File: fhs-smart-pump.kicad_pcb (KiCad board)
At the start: 2 copper layers, 92 x 87 mm, 27 parts, among them J1 Barrel_Jack_Switch, J2 Conn_01x02, J3 Screw_Terminal_01x02, J5 Screw_Terminal_01x07, K1 G5NB, K2 G5NB, Q1 2SA1015, Q2 2SA1015, U1 LM2596T-5, U2 PC817, U3 ESP32-C3_SUPERMINI_TH, U4 PC817

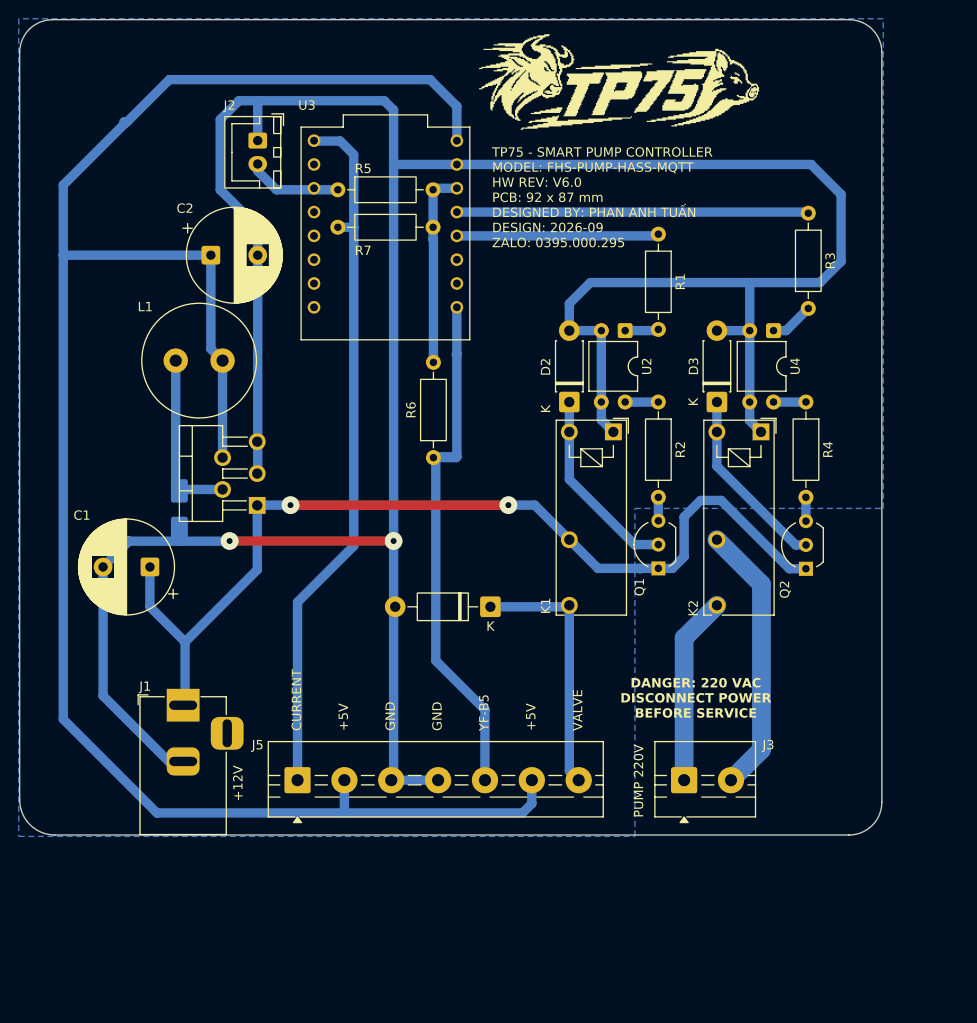
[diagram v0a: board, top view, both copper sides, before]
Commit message: cập nhật cơ khí pcb và báo cáo kiểm tra drc
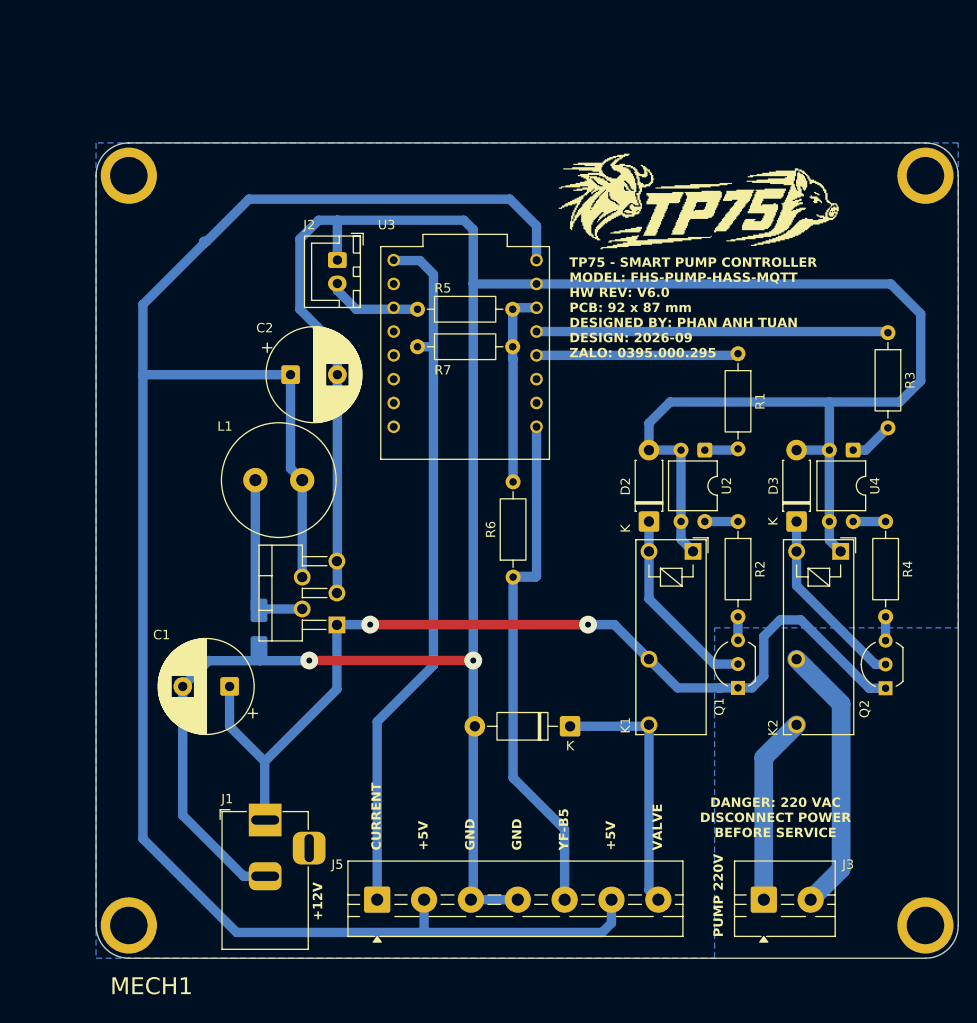
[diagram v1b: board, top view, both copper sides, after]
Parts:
- added MECH1: LK-PLC02_92x87, , F.Cu at (53.8, 150.0)
- moved ? 15.3 mm to (118.0, 69.2)
- moved C1 15.3 mm to (68.0, 121.0)
- moved C2 15.3 mm to (74.5, 87.7)
- moved D1 15.3 mm to (71.1, 114.9)
- moved D2 15.3 mm to (112.8, 103.4)
- moved D3 15.3 mm to (128.5, 103.4)
- moved D4 15.3 mm to (104.3, 125.2)
- moved J2 15.3 mm to (79.5, 75.5)
- moved J3 15.3 mm to (125.0, 143.8)
- moved J5 15.3 mm to (83.8, 143.8)
- moved K1 15.3 mm to (117.5, 106.6)
- moved L1 15.3 mm to (70.8, 99.0)
- moved Q1 15.3 mm to (122.2, 121.2)
- moved Q2 15.3 mm to (138.0, 121.2)
- moved R1 15.3 mm to (122.2, 85.5)
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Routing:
- net +12V: track 104.1 -> 103.5 mm
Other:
- outline, holes or cut-outs redrawn
- board text added: "TP75 - SMART PUMP CONTROLLER MODEL: FHS-PUMP-HASS-MQTT HW REV: V6.0 PCB: 92 x 87 mm DESIGNED BY: PHAN ANH TUAN DESIGN: 2026-09 ZALO: 0395.000.295"
- board text removed: "TP75 - SMART PUMP CONTROLLER MODEL: FHS-PUMP-HASS-MQTT HW REV: V6.0 PCB: 92 x 87 mm DESIGNED BY: PHAN ANH TUẤN DESIGN: 2026-09 ZALO: 0395.000.295"
